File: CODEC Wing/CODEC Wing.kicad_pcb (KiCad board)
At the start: 2 copper layers, 82 x 20.2 mm, 32 parts, among them J1 JACK_ST_2SW_PROPER, J2 JACK_ST_2SW_PROPER, U1 TL082, X1 CRYSTAL

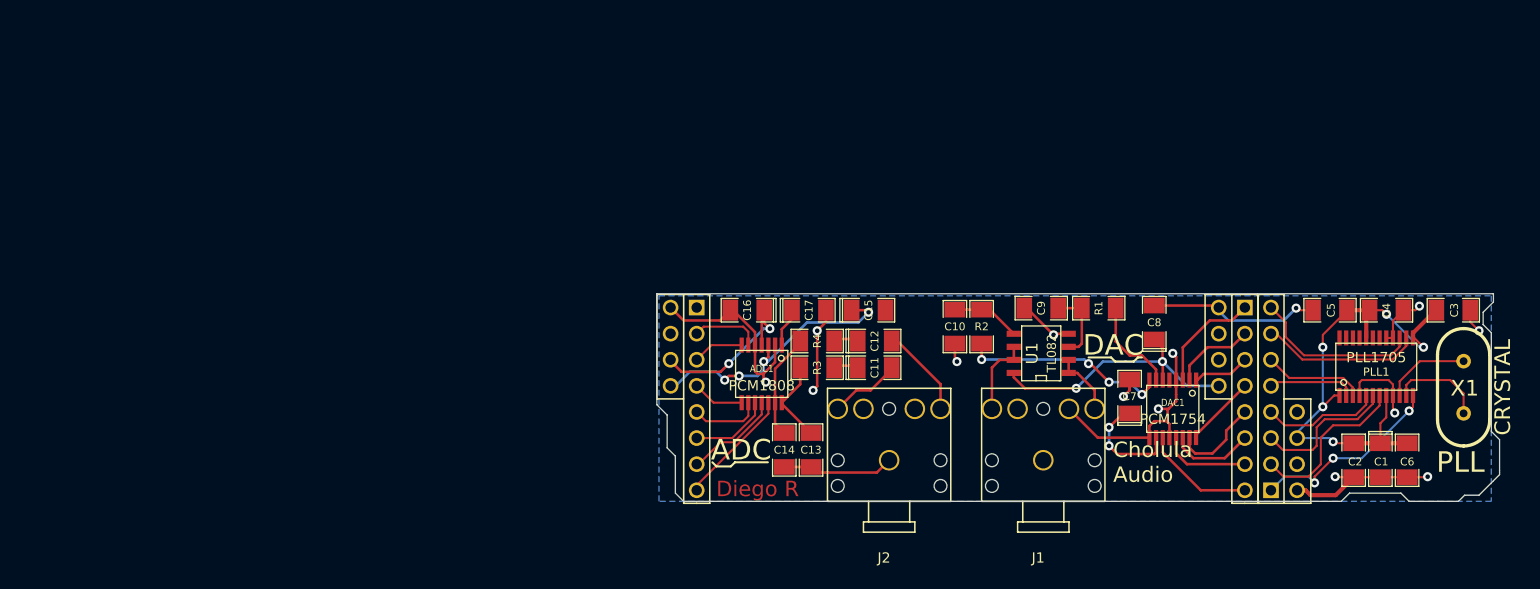
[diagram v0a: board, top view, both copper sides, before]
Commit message: More stuff
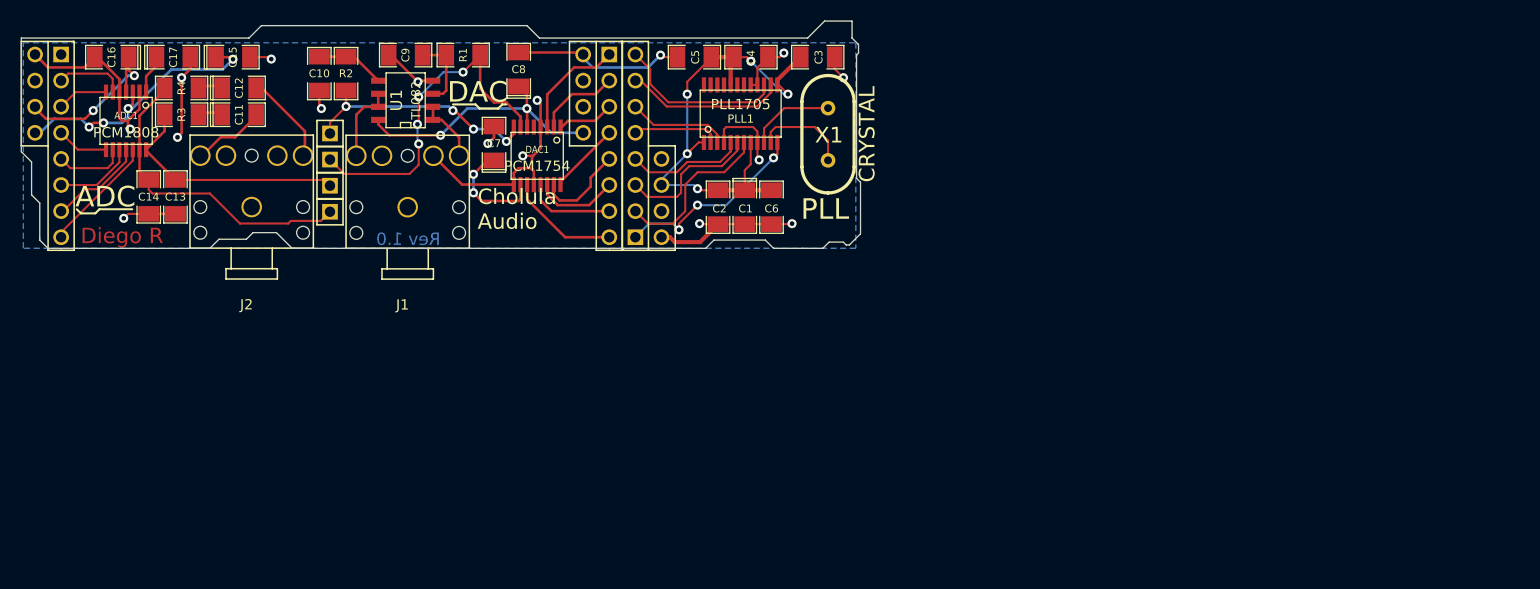
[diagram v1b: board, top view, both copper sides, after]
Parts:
- added TP1: CONN_1, PIN_ARRAY_1, F.Cu at (115.2, 84.3)
- added TP2: CONN_1, PIN_ARRAY_1, F.Cu at (115.2, 81.8)
- added TP3: CONN_1, PIN_ARRAY_1, F.Cu at (115.2, 86.9)
- added TP4: CONN_1, PIN_ARRAY_1, F.Cu at (115.2, 89.4)
- moved J2 66.7 mm to (107.6, 84.0)
- moved C1 66.6 mm to (155.6, 89.0)
- moved C14 66.6 mm to (97.6, 88.0)
- moved C16 66.6 mm to (94.0, 74.4)
- moved C17 66.6 mm to (100.0, 74.4)
- moved C2 66.6 mm to (153.0, 89.0)
- moved C3 66.6 mm to (162.7, 74.4)
- moved C4 66.6 mm to (156.2, 74.4)
- moved C5 66.6 mm to (150.7, 74.4)
- moved C6 66.6 mm to (158.2, 89.0)
- moved C7 66.6 mm to (131.2, 82.8)
- moved C8 66.6 mm to (133.6, 75.6)
- moved C9 66.6 mm to (122.6, 74.2)
- moved PAP1 66.6 mm to (89.0, 74.1)
- moved PAP2 66.6 mm to (142.4, 74.1)
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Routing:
- net N-0000037: track 9.33 -> 33.3 mm, vias 0 -> 4
- net N-0000052: track 10.3 -> 30.8 mm
- net N-0000051: track 8.47 -> 23.7 mm
- net GND: track 117.0 -> 113.4 mm, vias 14 -> 16
- net N-0000038: track 20.3 -> 23.5 mm
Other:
- board size 82 x 20.2 mm -> 81.7 x 22.1 mm
- board text added: "Rev 1.0"
